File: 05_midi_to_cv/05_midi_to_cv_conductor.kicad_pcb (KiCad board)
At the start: 2 copper layers, 40 x 100 mm, 33 parts, among them IC1 TLP2662, IC2 TLP2662, IC3 TLP2662, J1 MIDI IN 1, J2 MIDI IN 2, J3 MIDI IN 3, J4 AudioJack2, J5 Midi Fast Bus, J6 AudioJack2, J7 AudioJack2, U1 NCP1117-5.0_SOT223, U2 SN74HCT125

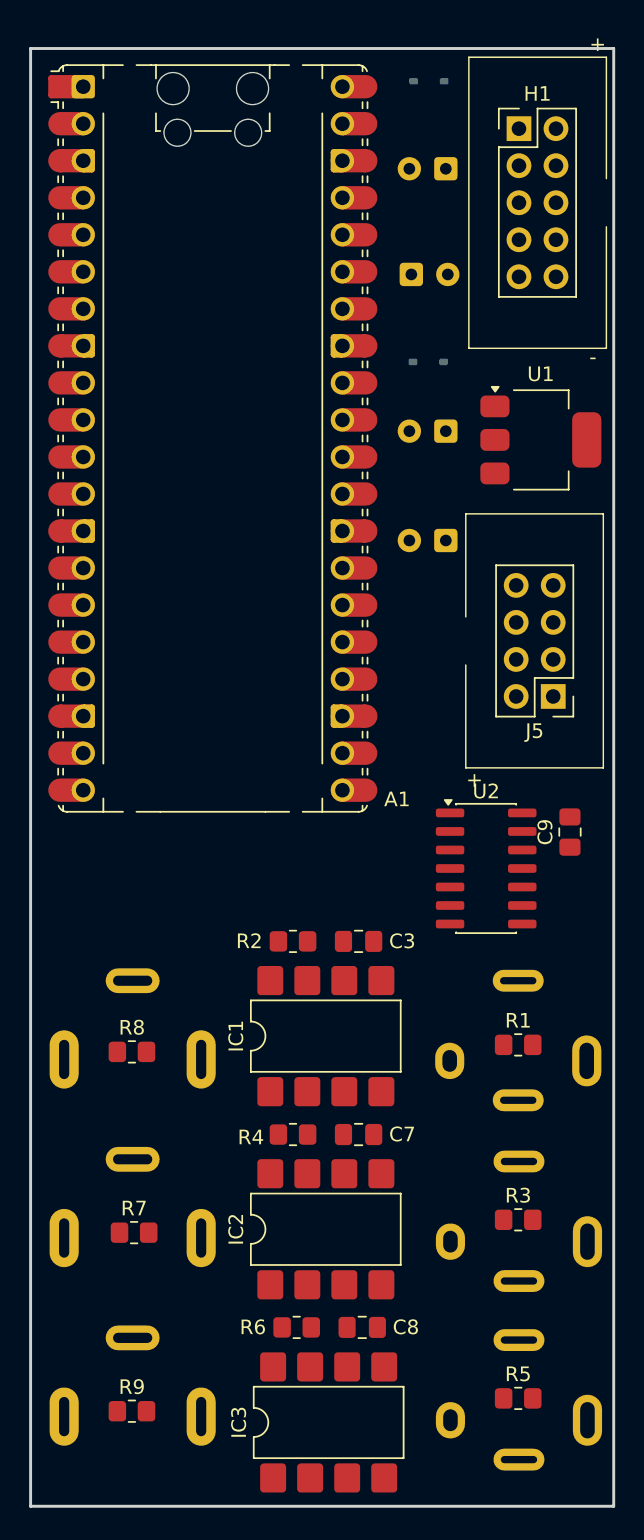
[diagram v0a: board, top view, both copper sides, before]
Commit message: updated 05
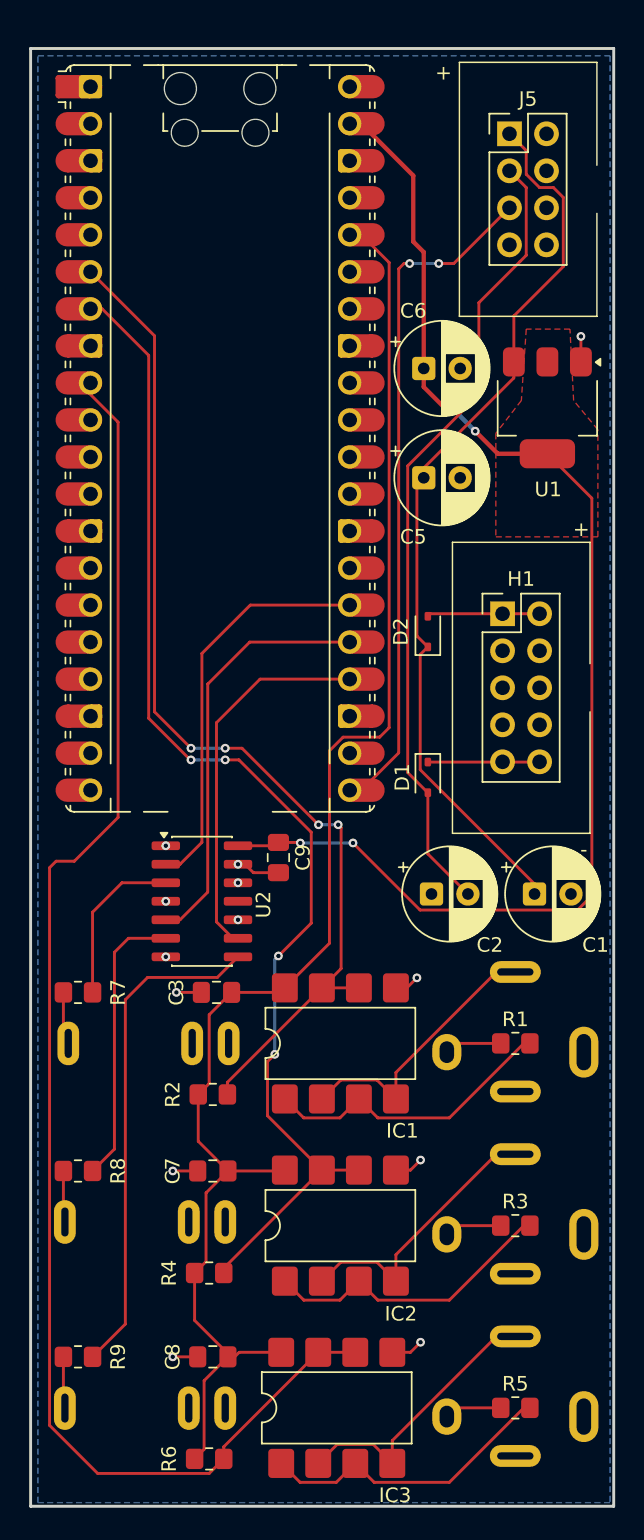
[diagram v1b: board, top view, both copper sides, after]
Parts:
- C1, C2, C5, C6, D1, D2: moved to F.Cu
- J4, J6, J7: value AudioJack2 -> ~; footprint cynthia:3.5mm jack mono -> cynthia:3.5mm thonk jack socket mono switched
- moved C1 50.1 mm to (58.3, 91.8), turned to 0 degrees
- moved C2 42.5 mm to (51.2, 91.8)
- moved J5 38.7 mm to (56.6, 39.6), turned to 0 degrees
- moved D2 37.8 mm to (51.0, 73.8), turned to 90 degrees
- moved H1 33.3 mm to (56.1, 72.5)
- moved D1 28.5 mm to (51.0, 83.8), turned to -90 degrees
- moved C9 20.1 mm to (40.8, 89.2), turned to -90 degrees
- moved U2 19.6 mm to (35.5, 92.2)
- moved R7 16.9 mm to (27.0, 98.5), turned to 180 degrees
- moved J4 12.8 mm to (30.7, 102.0), turned to -90 degrees
- moved R2 11.9 mm to (36.2, 105.5)
- moved J6 11.8 mm to (30.5, 114.2), turned to -90 degrees
- moved R4 11.1 mm to (36.0, 117.8)
- moved R6 10.8 mm to (36.0, 130.5)
- moved C8 10.4 mm to (36.2, 123.5), turned to 180 degrees
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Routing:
- net +3.3V: track 0.00 -> 105.0 mm
- net /midi input2/MIDI_IN: track 0.00 -> 101.6 mm
- net +5V: track 0.00 -> 88.5 mm, vias 0 -> 4
- net /midi input1/MIDI_IN: track 0.00 -> 83.7 mm, vias 0 -> 4
- net /midi input/MIDI_IN: track 0.00 -> 72.2 mm, vias 0 -> 4
- net +12V: track 0.00 -> 62.2 mm
- net -12V: track 0.00 -> 55.2 mm
- net MIDI_BUS: track 0.00 -> 46.2 mm, vias 0 -> 2
- net Net-(R9-Pad1): track 0.00 -> 34.4 mm
- net RUN: track 0.00 -> 28.9 mm
- net CLOCK: track 0.00 -> 27.6 mm
- net RESET: track 0.00 -> 26.0 mm
- net Net-(IC3-Pad1): track 0.00 -> 20.8 mm
- net Net-(IC1-Pad1): track 0.00 -> 20.5 mm
- net Net-(IC2-Pad1): track 0.00 -> 20.5 mm
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- added copper zone on F.Cu, net +5V
- added copper zone on B.Cu, net GND
